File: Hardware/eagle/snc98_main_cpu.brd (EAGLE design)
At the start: 168.2 x 30 mm, 89 parts, among them IC1 MCP170333MB, M1 IRLML2244, M12 IRLML2244, M2 IRLML2244, M3 IRLML2244, M4 IRLML6244, T1 BCR135, T2 BCR135, T3 BCR185, U1 74HC4051_MUX, U2 DS18B20, U3 ATMEGA1284P-PU, U4 TLV70033 / TC1185, Y2 12MHz

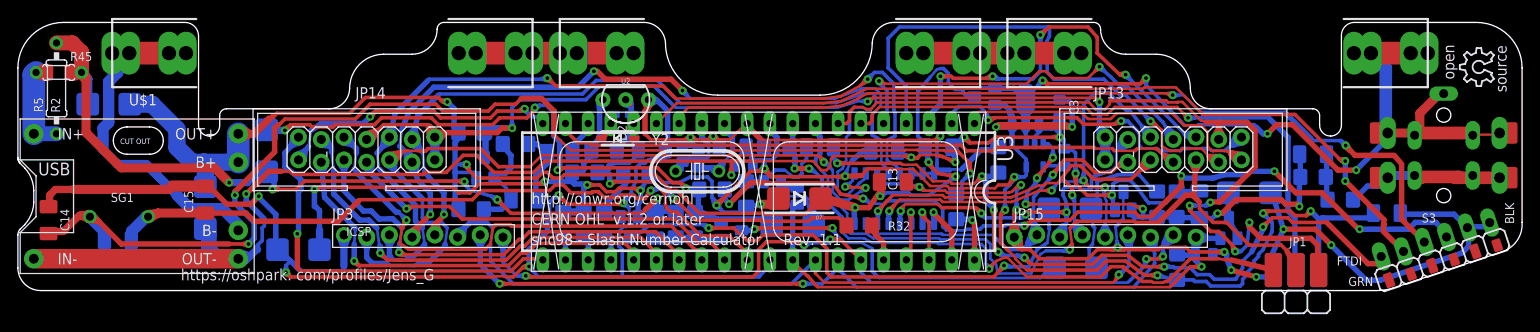
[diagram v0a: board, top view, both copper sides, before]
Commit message: cleanup_PCB
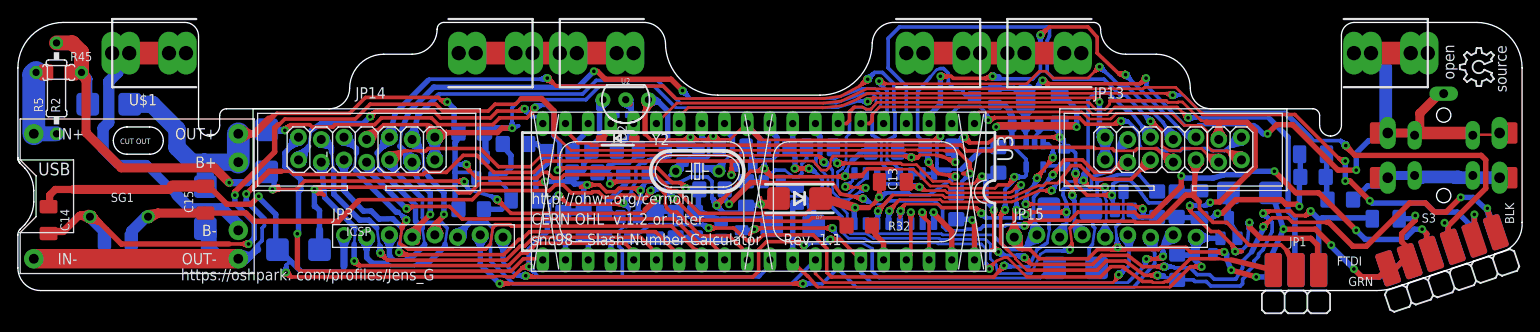
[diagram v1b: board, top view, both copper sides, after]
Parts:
- C3: value 220nF -> 1µ; device SparkFun:0805 -> rcl:C1206K
- moved JP6 5.07 mm to (147.7, -3.94)
- moved C2 0.65 mm to (146.3, 4.98)
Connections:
- net D8_RX0: now also JP6.P4, JP6.P4A; no longer JP6.3
- net D9_TX0: now also JP6.P5, JP6.P5A; no longer JP6.2
- net DTR: now also JP6.P6, JP6.P6A; no longer JP6.1
- net GND: now also C3.2; no longer C3.4
- net GND-ISO: now also JP6.P1, JP6.P1A, JP6.P2, JP6.P2A; no longer JP6.5, JP6.6
- net VCC: now also C3.1; no longer C3.3
- net VCC_IN: now also JP6.P3, JP6.P3A; no longer JP6.4
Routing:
- net CA_PWM: track 145.9 -> 891.1 mm
- net GND-ISO: track 392.2 -> 1017.8 mm, vias 17 -> 19
- net VCC: track 300.3 -> 855.5 mm
- net GND: track 215.9 -> 596.9 mm
- net DTR: track 103.3 -> 369.1 mm, vias 7 -> 9
- net V_IN: track 287.8 -> 528.4 mm
- net IO_DP: track 111.0 -> 350.0 mm
- net IO_A: track 76.5 -> 314.5 mm
- net A5: track 113.6 -> 341.5 mm
- net IO_C: track 62.2 -> 284.3 mm
- net IO_G: track 114.4 -> 295.9 mm
- net EN: track 66.6 -> 226.7 mm
- net D2_: track 64.5 -> 208.9 mm
- net D6_: track 103.5 -> 246.0 mm
- net IO_B: track 57.0 -> 194.9 mm
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
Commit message: cbrt_int96
cbrt added
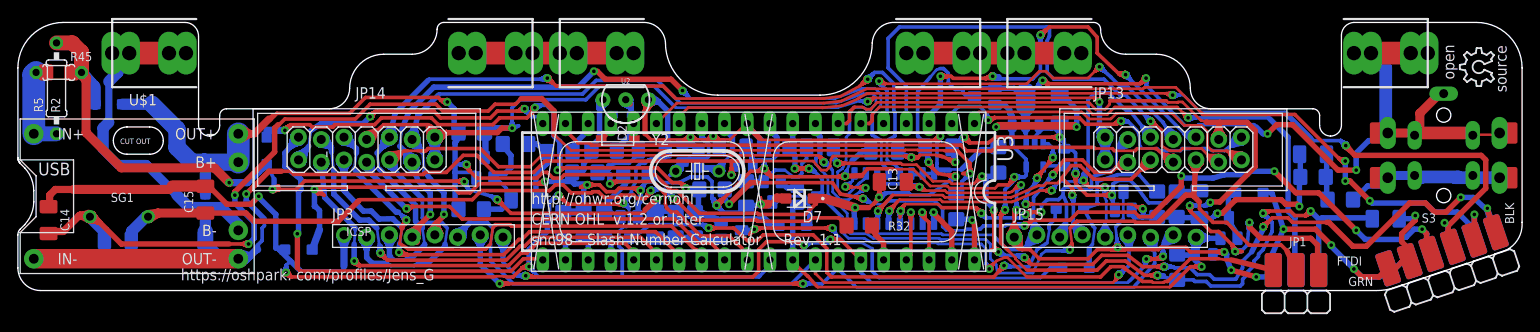
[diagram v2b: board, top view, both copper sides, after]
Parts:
- D10, D11, D12, D3, D4, D5, D7, D8, D9: device BaseApp:SMADIODE -> BaseApp:SOD-123F
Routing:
- net IO_C: track 284.3 -> 197.1 mm
- net VCC: track 855.5 -> 858.7 mm
- net VIN_P: track 183.5 -> 185.8 mm
- net GND-ISO: track 1017.8 -> 1019.8 mm
- net V_IN: track 528.4 -> 530.0 mm
- net CA_PWM2: track 95.2 -> 93.6 mm
- net IO_B: track 194.9 -> 196.4 mm
- net GND_POWER: track 5.48 -> 6.30 mm
- net GND: track 596.9 -> 597.7 mm
- net EN_: track 18.4 -> 19.1 mm
- net XX_3: track 163.6 -> 163.0 mm
